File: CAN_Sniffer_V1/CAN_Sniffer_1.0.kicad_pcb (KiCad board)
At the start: 2 copper layers, 99.1 x 99.2 mm, 51 parts, among them IC1 TPS2121RUXR, J1 USB_B_Micro, J2 MTJ-88ARX1-FSM-LG, J4 STL Link, J5 MEM2080-00-128-00-A, Q1 MMBT3906, Q4 MMBT3906, Q5 SQ2319CES-T1_GE3, U1 MCP2562, U2 AMS1117-3.3, U4 NUCLEO-F072RB, U5 TPS5430DDAR

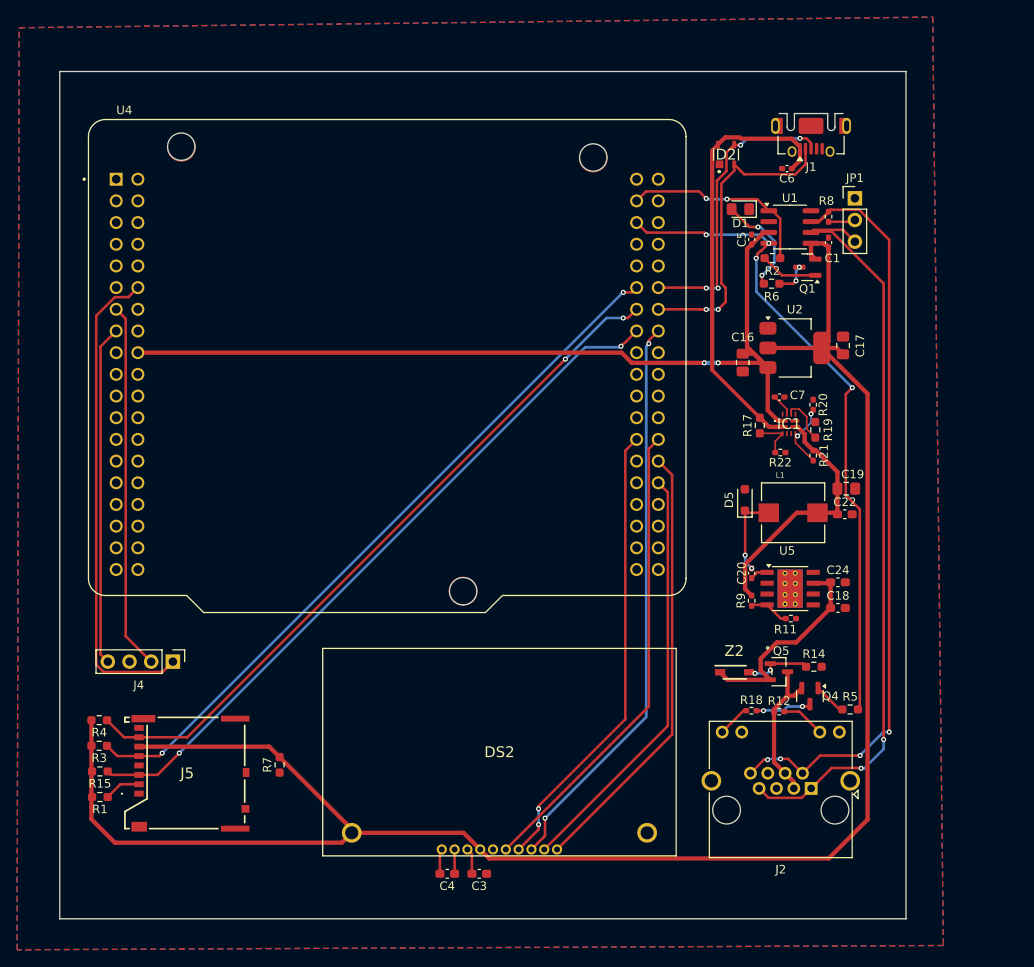
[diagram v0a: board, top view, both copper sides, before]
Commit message: iteration 2 routing
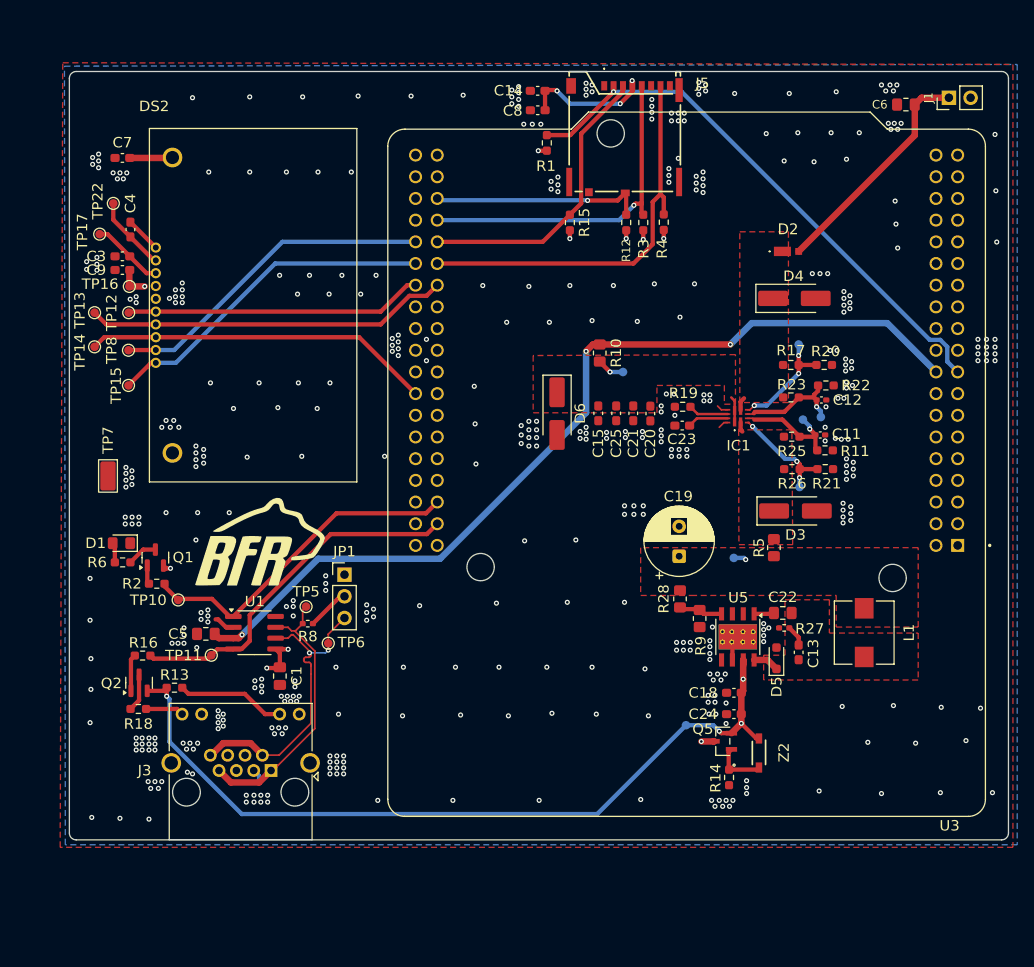
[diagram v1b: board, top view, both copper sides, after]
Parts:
- removed C16: 10u, Capacitor_SMD:C_0805_2012Metric_Pad1.18x1.45mm_HandSolder
- removed C17: 22u, Capacitor_SMD:C_0805_2012Metric_Pad1.18x1.45mm_HandSolder
- removed J2: MTJ-88ARX1-FSM-LG, Connector_RJ:RJ45_Amphenol_RJHSE538X
- removed J4: STL Link, Connector_PinHeader_2.54mm:PinHeader_1x04_P2.54mm_Vertical
- removed Q4: MMBT3906, Package_TO_SOT_SMD:SOT-23
- removed R7: 10k, Resistor_SMD:R_0603_1608Metric_Pad0.98x0.95mm_HandSolder
- removed U2: AMS1117-3.3, Package_TO_SOT_SMD:SOT-223-3_TabPin2
- removed U4: NUCLEO-F072RB, STM32F0_breakout:MODULE_NUCLEO-F072RB
- added C11: 100n, Capacitor_SMD:C_0402_1005Metric_Pad0.74x0.62mm_HandSolder, F.Cu at (144.8, 98.7)
- added C12: 100n, Capacitor_SMD:C_0402_1005Metric_Pad0.74x0.62mm_HandSolder, F.Cu at (145.0, 94.6)
- added C13: 470p, Capacitor_SMD:C_0603_1608Metric_Pad1.08x0.95mm_HandSolder, F.Cu at (142.3, 124.2)
- added C14: 10u, Capacitor_SMD:C_0603_1608Metric_Pad1.08x0.95mm_HandSolder, F.Cu at (111.7, 58.4)
- added C15: 10u, Capacitor_SMD:C_0603_1608Metric_Pad1.08x0.95mm_HandSolder, F.Cu at (118.8, 96.2)
- added C21: 4.7u, Capacitor_SMD:C_0603_1608Metric_Pad1.08x0.95mm_HandSolder, F.Cu at (122.9, 96.2)
- added C23: 100n, Capacitor_SMD:C_0603_1608Metric_Pad1.08x0.95mm_HandSolder, F.Cu at (128.7, 97.6)
- added C25: 10u, Capacitor_SMD:C_0603_1608Metric_Pad1.08x0.95mm_HandSolder, F.Cu at (120.9, 96.2)
- added C8: 100n, Capacitor_SMD:C_0603_1608Metric_Pad1.08x0.95mm_HandSolder, F.Cu at (111.7, 60.7)
- added C9: 100n, Capacitor_SMD:C_0603_1608Metric_Pad1.08x0.95mm_HandSolder, F.Cu at (63.1, 79.4)
- added D3: MBRA120ET3G, Diode_SMD:D_SMA_Handsoldering, F.Cu at (141.9, 107.6)
- added D4: MBRA120ET3G, Diode_SMD:D_SMA_Handsoldering, F.Cu at (141.8, 82.7)
- added D6: MBRA120ET3G, Diode_SMD:D_SMA_Handsoldering, F.Cu at (114.0, 96.2)
- added G***: LOGO, bfr_logos:BFR_Small, F.Cu at (79.2, 111.2)
- added J3: BRUHBus, Connector_RJ:RJ45_Amphenol_RJHSE538X, F.Cu at (80.5, 138.0)
- added Q2: MMBT3906, Package_TO_SOT_SMD:SOT-23, F.Cu at (65.0, 127.7)
- added R10: 0, Resistor_SMD:R_0805_2012Metric_Pad1.20x1.40mm_HandSolder, F.Cu at (119.0, 89.1)
- added R13: 3.3k, Resistor_SMD:R_0603_1608Metric_Pad0.98x0.95mm_HandSolder, F.Cu at (69.2, 128.3)
- added R16: 4.7k, Resistor_SMD:R_0603_1608Metric_Pad0.98x0.95mm_HandSolder, F.Cu at (65.5, 124.5)
- added R23: 27k, Resistor_SMD:R_0603_1608Metric_Pad0.98x0.95mm_HandSolder, F.Cu at (141.4, 94.3)
- added R25: 27k, Resistor_SMD:R_0603_1608Metric_Pad0.98x0.95mm_HandSolder, F.Cu at (141.5, 98.9)
- added R26: 10k, Resistor_SMD:R_0603_1608Metric_Pad0.98x0.95mm_HandSolder, F.Cu at (141.5, 102.7)
- added R27: 22, Resistor_SMD:R_0402_1005Metric_Pad0.72x0.64mm_HandSolder, F.Cu at (140.6, 121.3)
- added R28: 10k, Resistor_SMD:R_0805_2012Metric_Pad1.20x1.40mm_HandSolder, F.Cu at (128.4, 117.9)
- added TP1: VSUP-Filtered, TestPoint:TestPoint_Pad_D1.0mm, B.Cu at (129.1, 132.7)
- added TP10: TXD, TestPoint:TestPoint_Pad_D1.0mm, F.Cu at (69.6, 118.0)
- added TP11: RXD, TestPoint:TestPoint_Pad_D1.0mm, F.Cu at (73.5, 124.5)
- added TP12: LCD-SI, TestPoint:TestPoint_Pad_D1.0mm, F.Cu at (63.8, 84.4)
- added TP13: LCD-SCL, TestPoint:TestPoint_Pad_D1.0mm, F.Cu at (59.8, 84.4)
- added TP14: LCD-SCL, TestPoint:TestPoint_Pad_D1.0mm, F.Cu at (59.8, 88.4)
- added TP15: LCD-RST, TestPoint:TestPoint_Pad_D1.0mm, F.Cu at (63.8, 92.9)
- added TP16: LCD_3V3, TestPoint:TestPoint_Pad_D1.0mm, F.Cu at (63.9, 81.3)
- added TP17: LCD_VOUT, TestPoint:TestPoint_Pad_D1.0mm, F.Cu at (60.4, 75.2)
- added TP18: MUX-PR1, TestPoint:TestPoint_Pad_D1.0mm, B.Cu at (142.3, 88.1)
- added TP19: MUX-CP2, TestPoint:TestPoint_Pad_D1.0mm, B.Cu at (142.4, 104.8)
- added TP2: 5V-VSUP, TestPoint:TestPoint_Pad_D1.0mm, B.Cu at (134.7, 113.1)
- added TP20: MUX-OV1, TestPoint:TestPoint_Pad_D1.0mm, B.Cu at (144.9, 96.6)
- added TP21: MUX-OV2, TestPoint:TestPoint_Pad_D1.0mm, B.Cu at (142.8, 96.9)
- added TP22: LCD_3V3, TestPoint:TestPoint_Pad_D1.0mm, F.Cu at (62.0, 71.6)
- added TP4: 5V-MUX, TestPoint:TestPoint_Pad_D1.0mm, B.Cu at (121.7, 91.3)
- added TP5: CANH, TestPoint:TestPoint_Pad_D1.0mm, F.Cu at (84.6, 118.8)
- added TP6: CANL, TestPoint:TestPoint_Pad_D1.0mm, F.Cu at (87.2, 123.1)
- added TP7: GND, TestPoint:TestPoint_Keystone_5015_Micro_Mini, F.Cu at (61.4, 103.5)
- added TP8: LCD-RS, TestPoint:TestPoint_Pad_D1.0mm, F.Cu at (63.8, 88.8)
- added U3: NUCLEO-F072RB, STM32F0_breakout:MODULE_NUCLEO-F072RB, F.Cu at (129.2, 102.1)
- C1, C5, C6: footprint Capacitor_SMD:C_0402_1005Metric_Pad0.74x0.62mm_HandSolder -> Capacitor_SMD:C_0805_2012Metric_Pad1.18x1.45mm_HandSolder
- C19: value 47u -> 100u; footprint Capacitor_SMD:C_0805_2012Metric_Pad1.18x1.45mm_HandSolder -> Capacitor_THT:CP_Radial_D8.0mm_P3.50mm
- C20: value 10n -> 4.7u; footprint Capacitor_SMD:C_0402_1005Metric_Pad0.74x0.62mm_HandSolder -> Capacitor_SMD:C_0603_1608Metric_Pad1.08x0.95mm_HandSolder
- C22: value 22u -> 10n; footprint Capacitor_SMD:C_0603_1608Metric_Pad1.08x0.95mm_HandSolder -> Capacitor_SMD:C_0805_2012Metric_Pad1.18x1.45mm_HandSolder
- C7: footprint Capacitor_SMD:C_0402_1005Metric_Pad0.74x0.62mm_HandSolder -> Capacitor_SMD:C_0603_1608Metric_Pad1.08x0.95mm_HandSolder
- D2: value TPD2E001DZDR -> PD3S230LQ-7; footprint TPD2E001DZDR:TPD2E001DZDR -> PD3S230LQ-7:PD3S230LQ7
- J1: value USB_B_Micro -> Conn_01x02_Socket; footprint Connector_USB:USB_Micro-AB_Molex_47590-0001 -> Connector_PinHeader_2.54mm:PinHeader_1x02_P2.54mm_Vertical
- R11: value 3.3k -> 5.1k; footprint Resistor_SMD:R_0402_1005Metric_Pad0.72x0.64mm_HandSolder -> Resistor_SMD:R_0603_1608Metric_Pad0.98x0.95mm_HandSolder
- R12: value 3.3k -> 10k; footprint Resistor_SMD:R_0402_1005Metric_Pad0.72x0.64mm_HandSolder -> Resistor_SMD:R_0603_1608Metric_Pad0.98x0.95mm_HandSolder
- R18, R20, R22: footprint Resistor_SMD:R_0402_1005Metric_Pad0.72x0.64mm_HandSolder -> Resistor_SMD:R_0603_1608Metric_Pad0.98x0.95mm_HandSolder
- R21: value 10k -> 5.1k; footprint Resistor_SMD:R_0402_1005Metric_Pad0.72x0.64mm_HandSolder -> Resistor_SMD:R_0603_1608Metric_Pad0.98x0.95mm_HandSolder
- R5: value 4.7k -> 0; footprint Resistor_SMD:R_0603_1608Metric_Pad0.98x0.95mm_HandSolder -> Resistor_SMD:R_0805_2012Metric_Pad1.20x1.40mm_HandSolder
- R9: value 10k -> 3.3k; footprint Resistor_SMD:R_0402_1005Metric_Pad0.72x0.64mm_HandSolder -> Resistor_SMD:R_0805_2012Metric_Pad1.20x1.40mm_HandSolder
- moved R1 92.8 mm to (112.8, 64.5), turned to -90 degrees
- moved J5 90.7 mm to (121.9, 63.4), turned to 0 degrees
- moved R3 88.4 mm to (124.1, 73.8), turned to -90 degrees
- moved R4 88.2 mm to (126.5, 73.8), turned to -90 degrees
- moved R15 84.6 mm to (115.5, 73.8), turned to -90 degrees
- moved C4 84.1 mm to (64.0, 74.6), turned to 90 degrees
- moved Q1 83.6 mm to (67.0, 113.1), turned to 90 degrees
- moved C3 83.5 mm to (63.1, 77.8), turned to 0 degrees
- moved R6 82.7 mm to (63.1, 113.6)
- moved D1 82.4 mm to (63.0, 111.4)
- moved C7 81.9 mm to (63.1, 66.2), turned to 180 degrees
- moved C1 81.9 mm to (81.5, 126.9), turned to -90 degrees
- moved R2 81.6 mm to (67.1, 116.1)
- moved C5 78.9 mm to (72.9, 122.0), turned to 180 degrees
- moved U1 78.7 mm to (78.6, 121.9)
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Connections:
- net /CAN1H renamed /CAN+
- net /CAN1L renamed /CAN-
- net /CAN1_TX renamed /CAN_TX
- net /Power/24V-5V-Buck-Converter/VSUP renamed /Power/VSUP_Filtered
- net /SD-CS renamed /SD_CS
- net /SD-MISO renamed /SD_MISO
- net /SD-MOSI renamed /SD_MOSI
- net /SD-SCK renamed /SD_SCK
- net Net-(DS2-C1+) renamed /LCD_C1
- net Net-(DS2-VOUT) renamed /LCD_VOUT
- C19 pad 1: /Power/24V-5V-Buck-Converter/5V-VSUP -> Net-(C19-Pad1)
- C20 pad 1: Net-(U5-BOOT) -> Net-(D6-K)
- C20 pad 2: Net-(D5-K) -> GND
- C22 pad 1: /Power/24V-5V-Buck-Converter/5V-VSUP -> Net-(U5-BOOT)
- C22 pad 2: GND -> Net-(D5-K)
- C6 pad 1: /Power/Power-Mux/VBUS -> /U5V-IN
- C7 pad 1: Net-(IC1-SS) -> +3.3V
- D2 pad 1: GND -> Net-(D2-K)
- D2 pad 2: /USB_DM -> /U5V-IN
- IC1 pad 1: +5V -> Net-(D6-K)
- IC1 pad 2: /Power/Power-Mux/VBUS -> /Power/24V-5V-Buck-Converter/5V_VSUP
- IC1 pad 4: unconnected-(IC1-OV2-Pad4) -> Net-(IC1-OV2)
- IC1 pad 5: unconnected-(IC1-OV1-Pad5) -> Net-(IC1-OV1)
- IC1 pad 7: /Power/24V-5V-Buck-Converter/5V-VSUP -> Net-(D2-K)
- IC1 pad 8: unconnected-(IC1-OUT_2-Pad8) -> Net-(D6-K)
- J1 pad 1: /Power/Power-Mux/VBUS -> /U5V-IN
- J1 pad 2: /USB_DM -> unconnected-(J1-Pin_2-Pad2)
- J5 pad 4: GND -> +3.3V
- J5 pad 6: +3.3V -> GND
- J5 pad DSW2: /SD-CD -> /SD_CD
- L1 pad 2: /Power/24V-5V-Buck-Converter/5V-VSUP -> Net-(C19-Pad1)
- R11 pad 2: Net-(U5-VSENSE) -> Net-(IC1-OV2)
- R12 pad 1: Net-(J2-Pad10) -> /SD_CD
- R12 pad 2: /Power/RJ45-connector/VSUP -> +3.3V
- R17 pad 1: Net-(IC1-CP2) -> Net-(IC1-PR1)
- R17 pad 2: /Power/Power-Mux/VBUS -> Net-(D2-K)
- R21 pad 1: Net-(IC1-PR1) -> GND
- R21 pad 2: /Power/24V-5V-Buck-Converter/5V-VSUP -> Net-(IC1-CP2)
- R22 pad 2: Net-(IC1-CP2) -> Net-(IC1-OV1)
- R5 pad 1: /CAN1_RX -> Net-(C19-Pad1)
- R5 pad 2: Net-(Q4-B) -> /Power/24V-5V-Buck-Converter/5V_VSUP
- R9 pad 1: Net-(U5-VSENSE) -> GND
- R9 pad 2: /Power/24V-5V-Buck-Converter/5V-VSUP -> Net-(U5-VSENSE)
- U1 pad 4: /CAN1_RX -> /CAN_RX
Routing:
- net +3.3V: track 219.6 -> 37.8 mm, vias 0 -> 12
- net /CAN1_RX: track 77.5 -> 0.00 mm, vias 4 -> 0
- net /Power/VSUP_Filtered: track 24.9 -> 95.5 mm, vias 0 -> 4
- net /SD_CS: track 4.30 -> 65.5 mm, vias 0 -> 1
- net /CAN+: track 91.1 -> 32.7 mm, vias 4 -> 0
- net /STM-Nucleo/NRST: track 56.9 -> 0.00 mm
- net /CAN-: track 88.9 -> 36.3 mm
- net /Power/Power-Mux/VBUS: track 51.1 -> 0.00 mm
- net /SD_MOSI: track 83.7 -> 34.5 mm, vias 2 -> 0
- net /SD_SCK: track 85.3 -> 39.9 mm, vias 2 -> 1
- net /STM-Nucleo/SWDIO: track 43.0 -> 0.00 mm
- net /CAN_RX: track 0.00 -> 42.1 mm
- net /STM-Nucleo/SWCLK: track 39.8 -> 0.00 mm
- net /USB_DM: track 36.3 -> 0.00 mm, vias 2 -> 0
- net /SD_MISO: track 83.6 -> 47.6 mm, vias 2 -> 0
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- added copper zone on In2.Cu, net +3.3V
- added copper zone on F.Cu, net /Power/24V-5V-Buck-Converter/5V_VSUP
- added copper zone on In2.Cu, net /Power/RJ45-connector/VSUP
- added copper zone on In2.Cu, net /Power/VSUP_Filtered
- added copper zone on In1.Cu, net GND
- added copper zone on F.Cu, net Net-(C19-Pad1)
- added copper zone on F.Cu, net Net-(D2-K)
- added copper zone on F.Cu, net Net-(D5-K)
- added copper zone on F.Cu, net Net-(D6-K)
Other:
- board size 99.1 x 99.2 mm -> 110 x 90 mm
- copper layers 2 -> 4
